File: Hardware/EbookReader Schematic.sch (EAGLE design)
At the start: 103 parts, among them IC1 BD5229G-TR, IC4 XC6220A331MR-G, J1 FH34SRJ-24S-0.5SH_99_, J2 SAMACSYS_PARTS_USB4110-GF-A, J3 QWIIC_RIGHT_ANGLE, J4 112A-TAAR-R03_ATTEND, Q1 20V/4.2A/52mΩ/1.4W, Q2 20V/4.2A/52mΩ/1.4W, Q3 SI1308EDL-T1-GE3, U1 W25Q512JVEIQ, U2 ESP32-C6-WROOM-1-N8, U3 DS3231SN#, U4 MAX17048G+T10

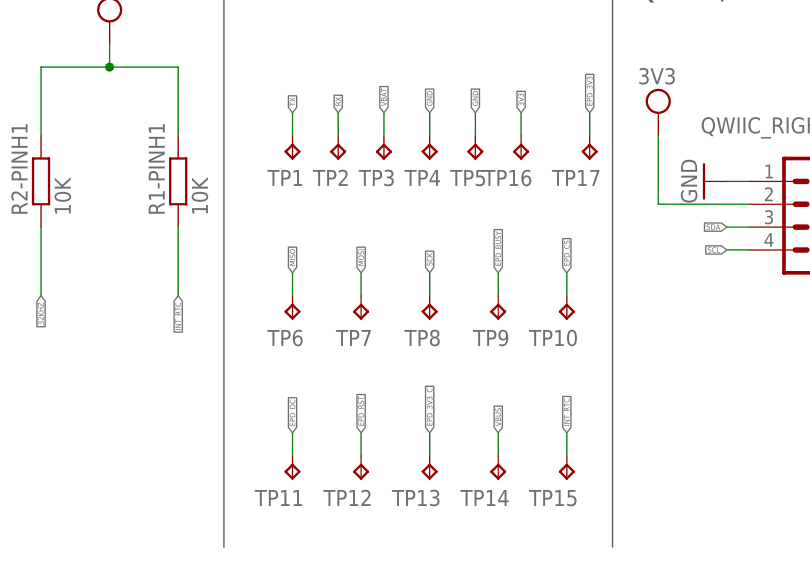
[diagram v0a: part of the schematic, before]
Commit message: Incarcare versiuni finale PCB (2D si 3D)
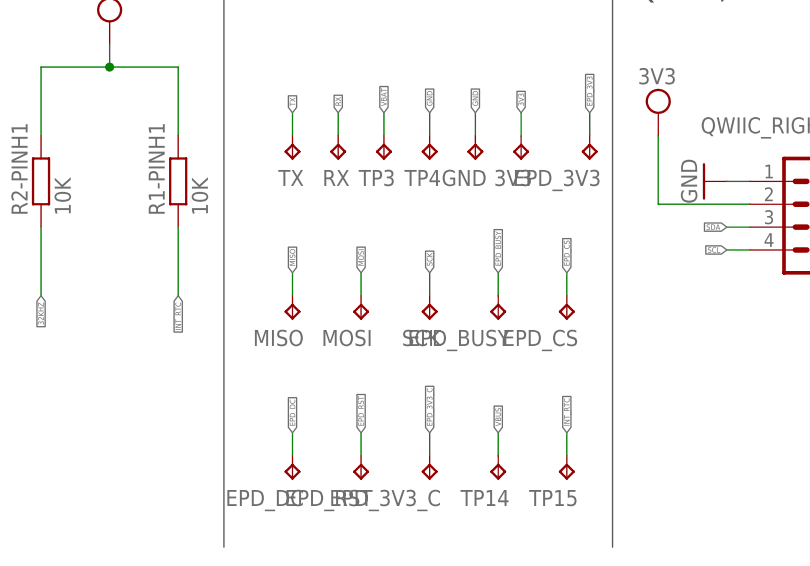
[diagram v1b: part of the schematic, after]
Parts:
- L1: device DeskAssistant v19 v1:744043680IND_4828-WE-TPC_WRE -> DeskAssistant v19 v1:744043680IND_4828-WE-TPC_WRE2
- renumbered TP1 to TX, TP10 to EPD_CS, TP11 to EPD_DC, TP12 to EPD_RST, TP13 to EPD_3V3_C, TP16 to 3V3, TP17 to EPD_3V3, TP2 to RX, TP5 to GND, TP6 to MISO, TP7 to MOSI, TP8 to SCK, TP9 to EPD_BUSY
